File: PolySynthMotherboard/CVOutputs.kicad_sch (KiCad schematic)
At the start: 168 parts, among them U301 DAC7578xPW, U302 TL074, U303 TL072, U304 TMUX4051, U305 TL074, U306 TMUX4051, U307 TL074, U308 TMUX4051, U309 TMUX4051, U310 TL074, U311 TL074, U312 TL074, U313 TMUX4051, U314 TL074, U315 TL074, U316 TL074, U317 TMUX4051, U318 TMUX4051, U319 TL074, U320 TL074

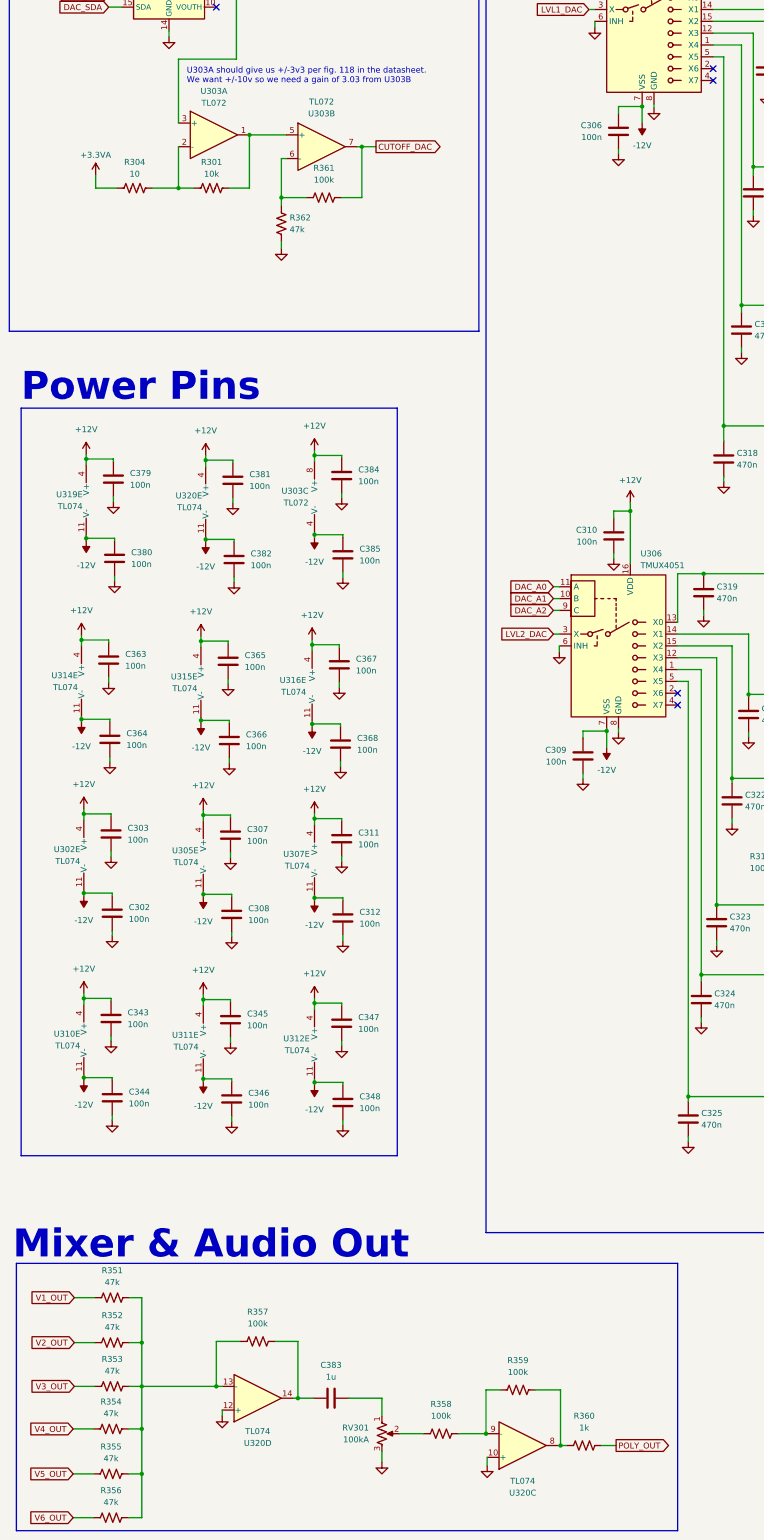
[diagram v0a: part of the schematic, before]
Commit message: power supply/ output circuits
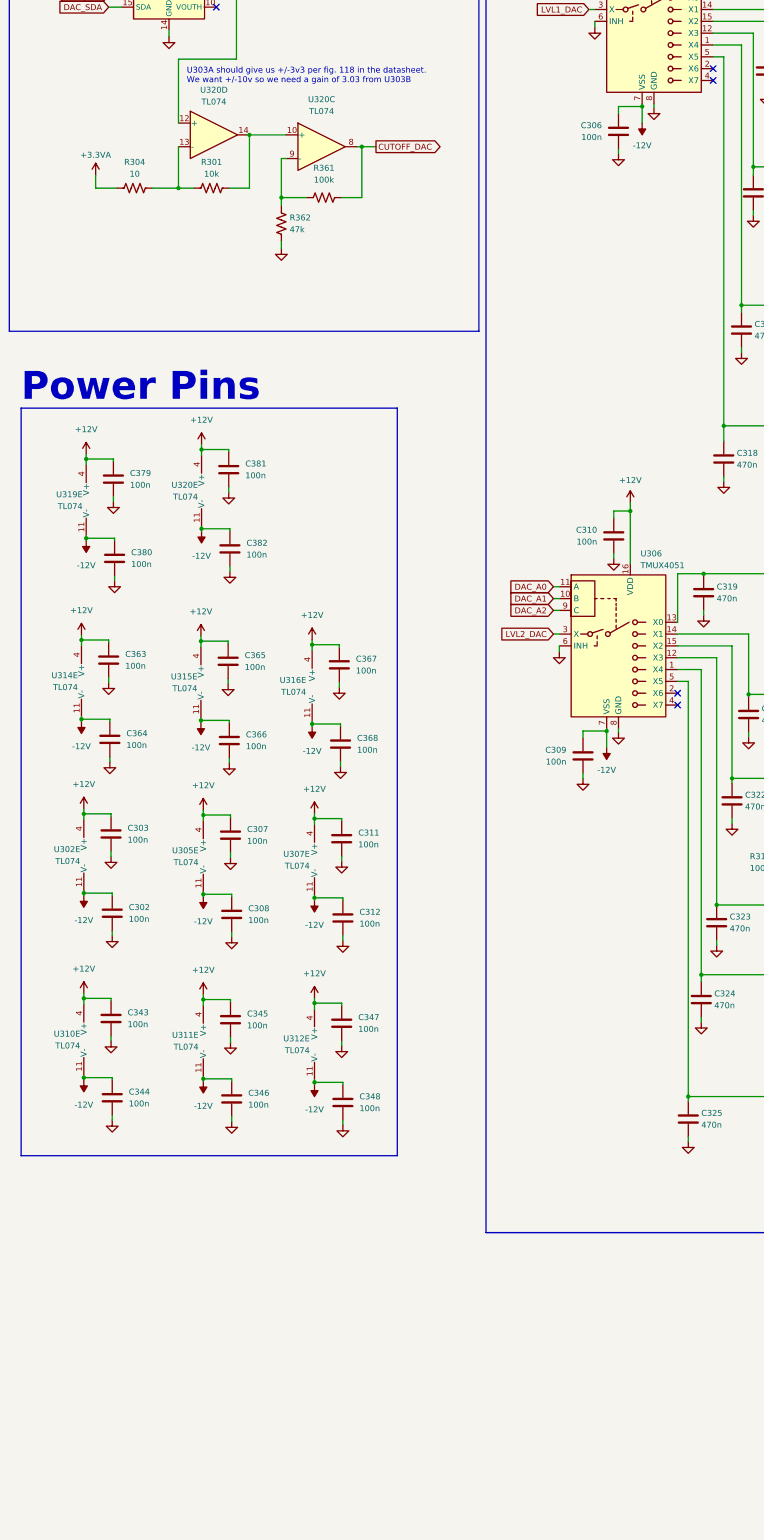
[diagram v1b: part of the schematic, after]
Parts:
- removed C383: 1u, symbol Device:C
- removed C384, C385: 100n, symbol Device:C
- removed R351, R352, R353, R354, R355, R356: 47k, symbol Device:R_US
- removed R357, R358, R359: 100k, symbol Device:R_US
- removed R360: 1k, symbol Device:R_US
- removed RV301: 100kA, symbol Device:R_Potentiometer_US
- removed U303: TL072, symbol Amplifier_Operational:TL072
- C301, C302, C303, C304, C305, C306, C307, C308, C309, C310, C311, C312, C313, C314, C315, C316, C317, C318, C319, C320, C321, C322, C323, C324, C325, C326, C327, C328, C329, C330, C331, C332, C333, C334, C335, C336, C337, C338, C339, C340, C341, C342, C343, C344, C345, C346, C347, C348, C349, C350, C351, C352, C353, C354, C355, C356, C357, C358, C359, C360, C361, C362, C363, C364, C365, C366, C367, C368, C369, C370, C371, C372, C373, C374, C375, C376, C377, C378, C379, C380, C381, C382: footprint (none) -> Capacitor_SMD:C_0805_2012Metric
- R301, R302, R303, R304, R305, R306, R307, R308, R309, R310, R311, R312, R313, R314, R315, R316, R317, R318, R319, R320, R321, R322, R323, R324, R325, R326, R327, R328, R329, R330, R331, R332, R333, R334, R335, R336, R337, R338, R339, R340, R341, R342, R343, R344, R345, R346, R347, R348, R349, R350, R361, R362: footprint (none) -> PCM_Resistor_SMD_AKL:R_0805_2012Metric
- U302, U305, U307, U310, U311, U312, U314, U315, U316, U319, U320: footprint (none) -> PCM_Package_SO_AKL:SOIC-14_3.9x8.7mm_P1.27mm
- U304, U306, U308, U309, U313, U317, U318: footprint (none) -> Package_SO:TSSOP-16_4.4x5mm_P0.65mm
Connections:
- net CUTOFF_DAC: now also U320.8
- net GND: no longer U320.10 (+), U320.12 (+)
- net at R301.2: now also U320.10 (+), U320.14
- net at R361.1, R362.2: now also U320.9 (-)
- net at U320.13 (-): now also R301.1, R304.2
- net at U301.7 (VOUTG): now also U320.12 (+)
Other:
- note removed: "Mixer & Audio Out"
- moved on the sheet: U320C, U320D
